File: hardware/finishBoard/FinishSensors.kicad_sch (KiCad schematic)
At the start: 11 parts, among them U2 7414

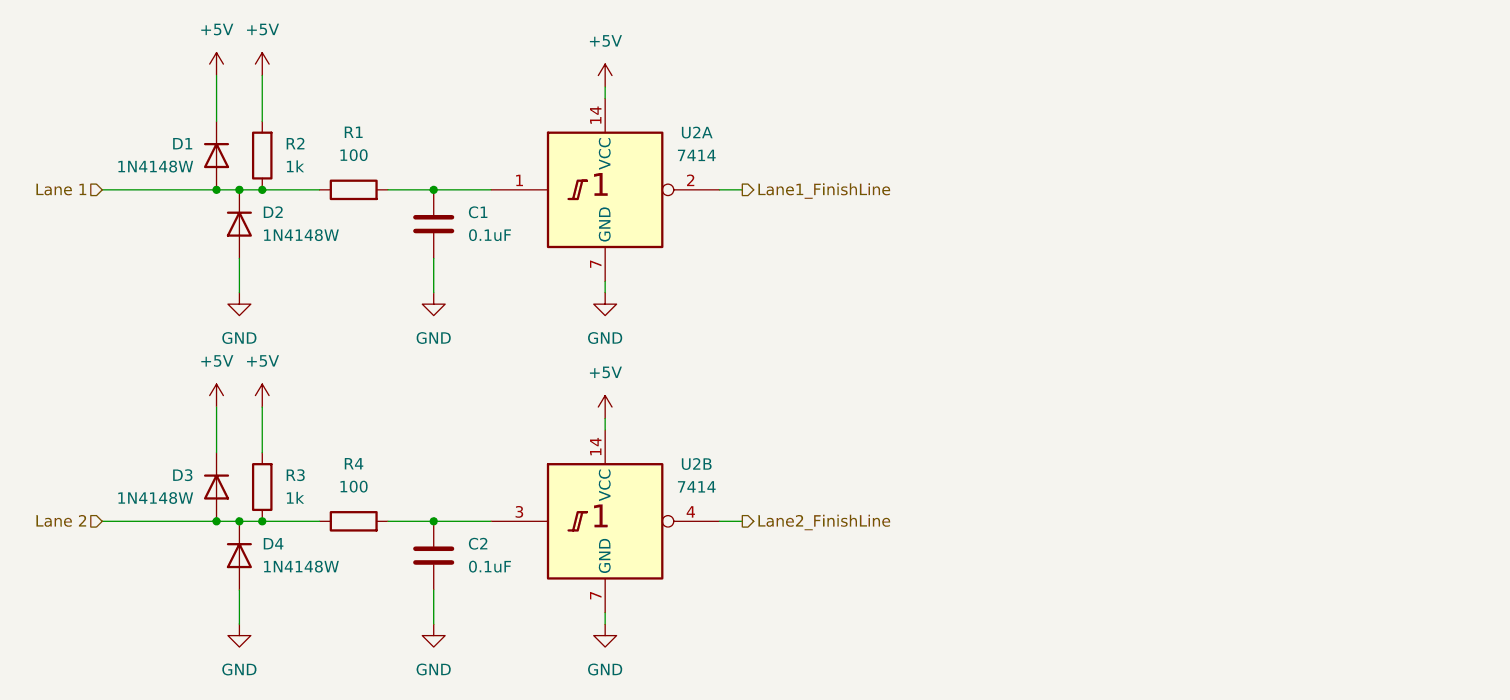
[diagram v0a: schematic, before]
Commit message: Finish Control Board completion for order
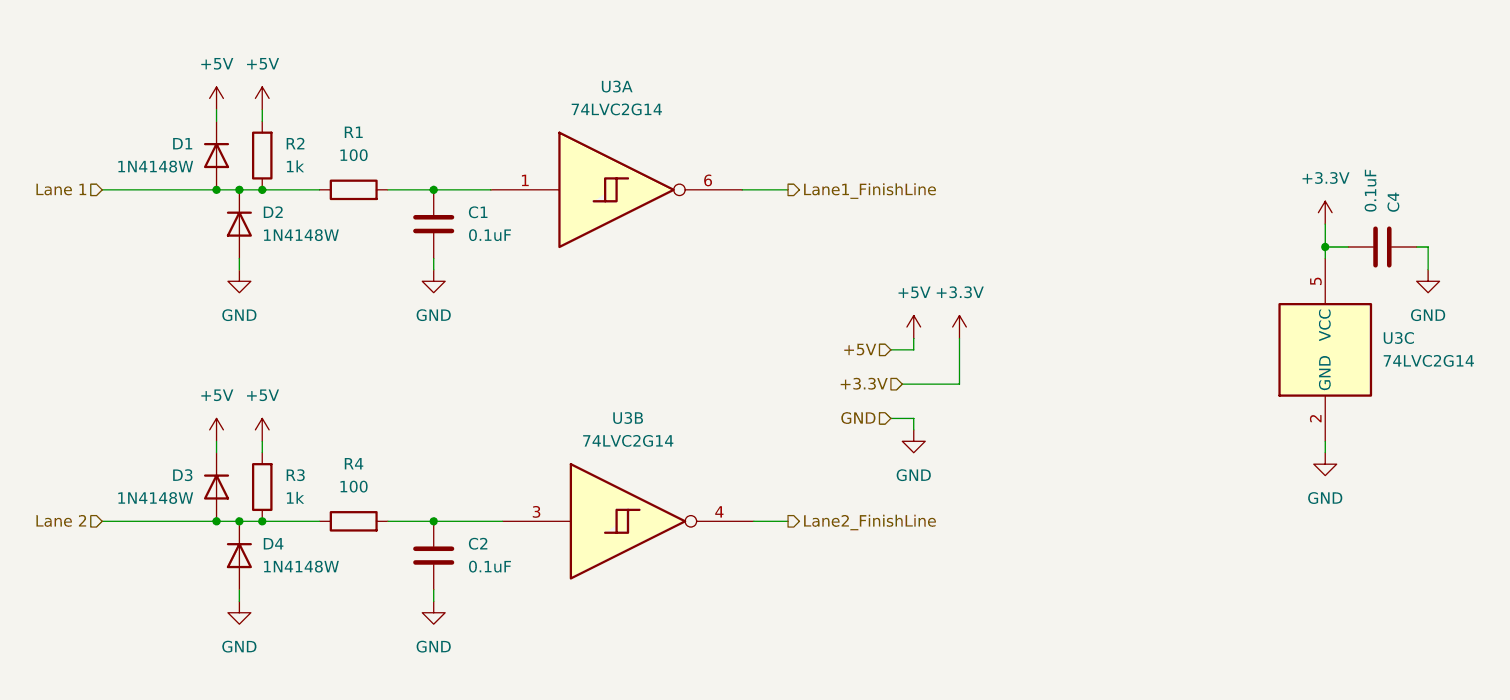
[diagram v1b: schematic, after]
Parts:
- removed U2: 7414, Package_SO:SOIC-14_3.9x8.7mm_P1.27mm, symbol 74xx_IEEE:7414
- added C4: 0.1uF, Capacitor_SMD:C_0805_2012Metric, symbol Device:C
- added U3: 74LVC2G14, Package_TO_SOT_SMD:SOT-23-6_Handsoldering, symbol 74xGxx:74LVC2G14
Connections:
- net GND: now also C4.1, U3.2 (GND)
- net Lane1_FinishLine: now also U3.6
- net Lane2_FinishLine: now also U3.4
- net at C1.1, R1.2: now also U3.1
- net at C2.1, R4.2: now also U3.3
- new net +3.3V: C4.2, U3.5 (VCC)
